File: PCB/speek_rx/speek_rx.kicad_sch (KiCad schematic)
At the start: 24 parts, among them U1 ESP32-D0WD-V3, U2 W25Q32JVSSIQ_C179173, X1 XL2EL89CPI-111YLC-40M

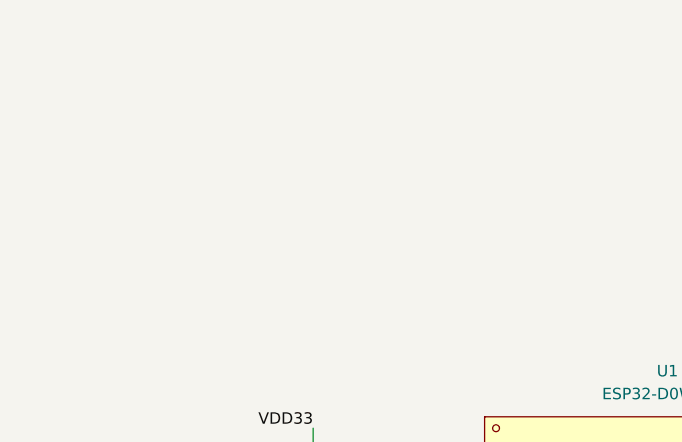
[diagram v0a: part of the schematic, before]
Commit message: finishs
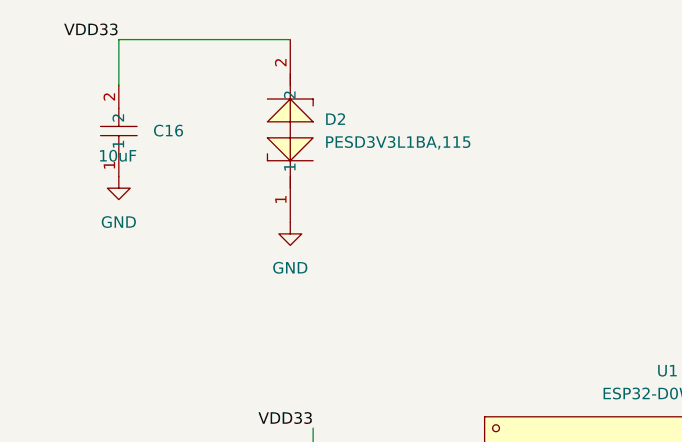
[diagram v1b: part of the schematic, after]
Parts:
- added C16: 10uF, lcsc:C0402, symbol lcsc:CL05A106MP5NUNC_C15525
- added D2: PESD3V3L1BA,115, easyeda2kicad:SOD-323_L1.7-W1.3-LS2.5-BI-1, symbol lcsc:PESD3V3L1BA,115
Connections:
- net GND: now also C16.1, D2.1
- net VDD33: now also C16.2, D2.2

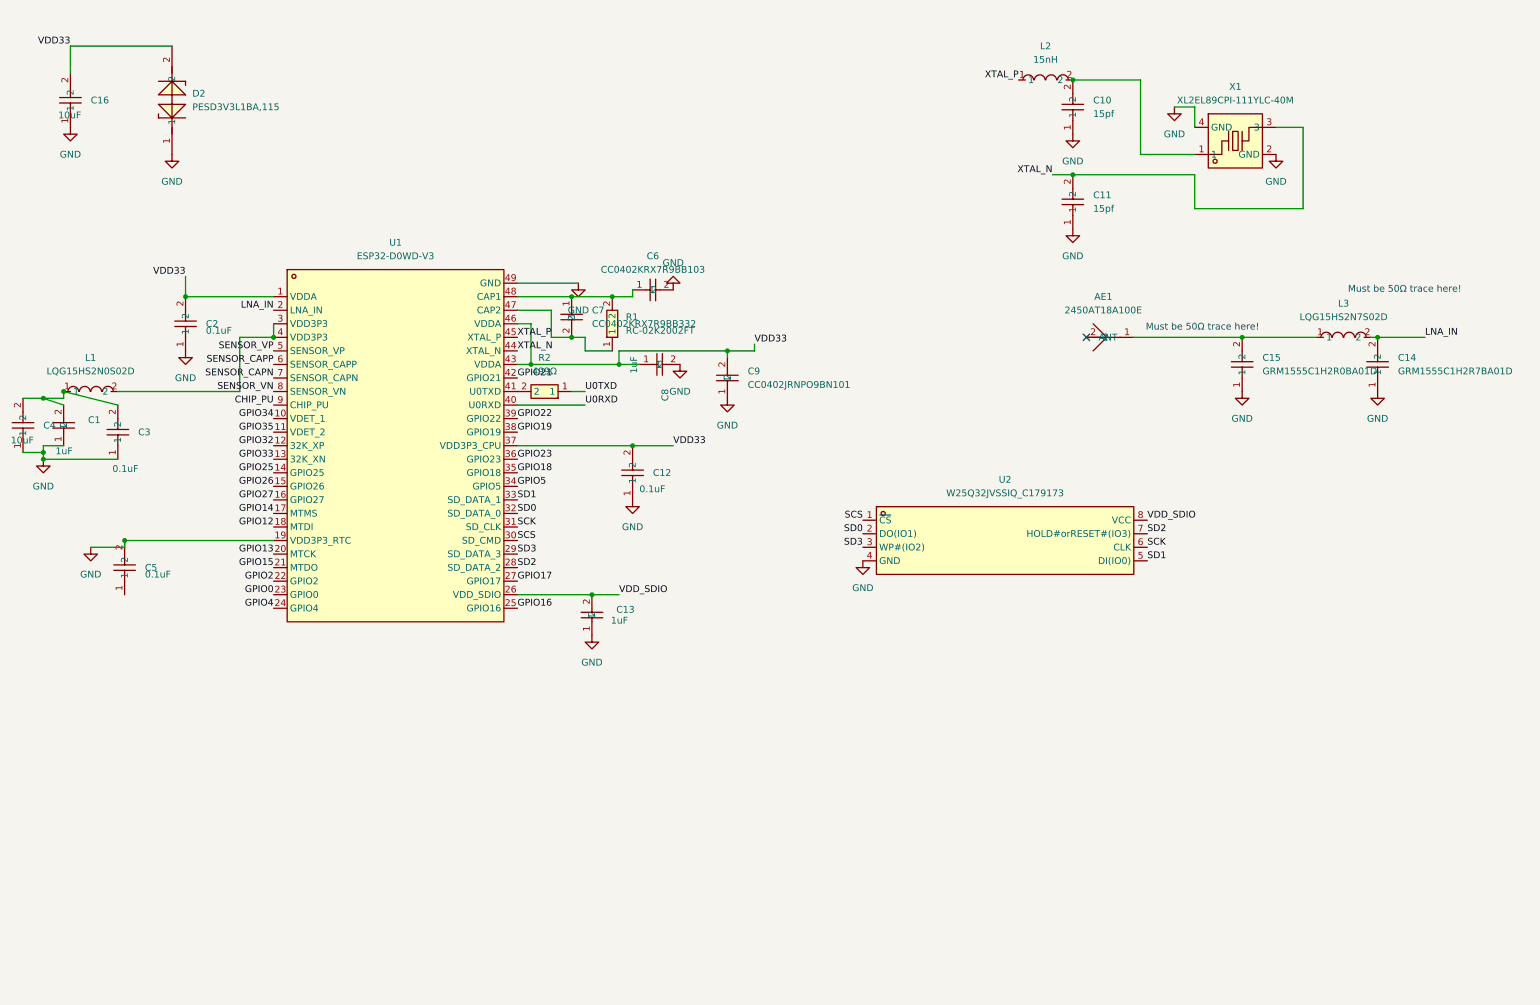
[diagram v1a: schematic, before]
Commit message: ldo, strappings, uart, USB
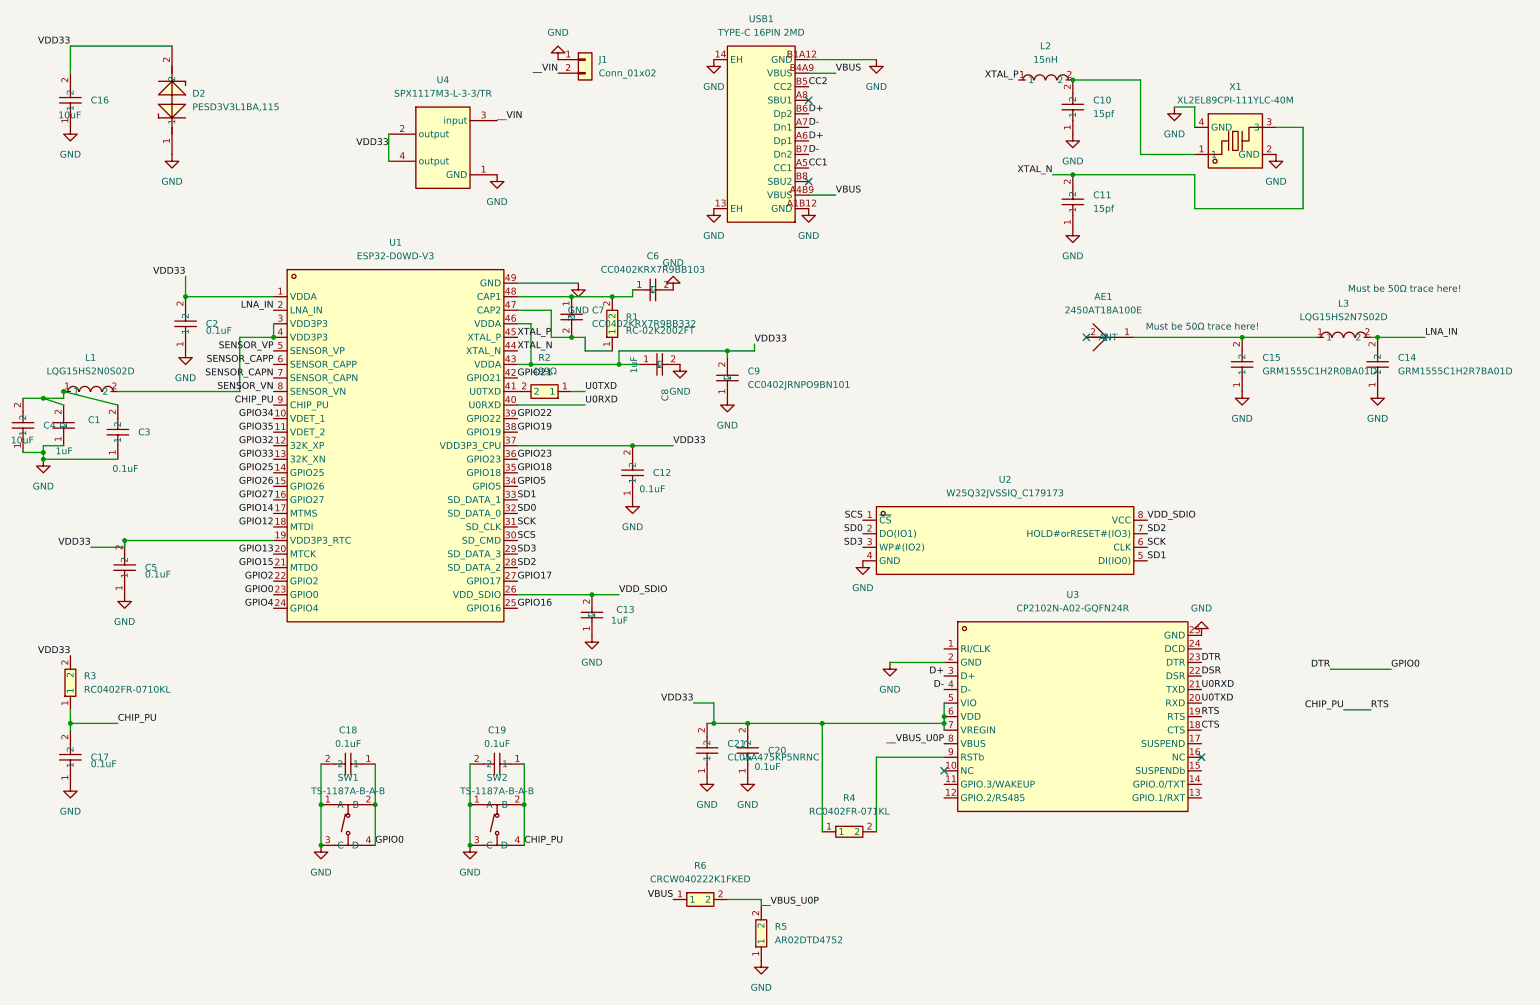
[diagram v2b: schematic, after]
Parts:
- added C17, C18, C19, C20: 0.1uF, lcsc:C0402, symbol lcsc:CC0402KRX7R7BB104
- added C21: CL05A475KP5NRNC, easyeda2kicad:C0402, symbol lcsc:CL05A475KP5NRNC
- added J1: Conn_01x02, symbol Connector_Generic:Conn_01x02
- added R3: RC0402FR-0710KL, easyeda2kicad:R0402, symbol lcsc:RC0402FR-0710KL
- added R4: RC0402FR-071KL, easyeda2kicad:R0402, symbol lcsc:RC0402FR-071KL
- added R5: AR02DTD4752, easyeda2kicad:R0402, symbol lcsc:AR02DTD4752
- added R6: CRCW040222K1FKED, easyeda2kicad:R0402, symbol lcsc:CRCW040222K1FKED
- added SW1, SW2: TS-1187A-B-A-B, easyeda2kicad:SW-SMD_4P-L5.1-W5.1-P3.70-LS6.5-TL_H1.5, symbol lcsc:TS-1187A-B-A-B
- added U3: CP2102N-A02-GQFN24R, easyeda2kicad:QFN-24_L4.0-W4.0-P0.50-TL-EP2.6, symbol lcsc:CP2102N-A02-GQFN24R
- added U4: SPX1117M3-L-3-3/TR, easyeda2kicad:SOT-223-4_L6.5-W3.5-P2.30-LS7.0-BR, symbol lcsc:SPX1117M3-L-3-3_TR
- added USB1: TYPE-C 16PIN 2MD, lcsc:USB-C-SMD_TYPE-C-16PIN-2MD-073, symbol lcsc:TYPE-C16PIN2MD
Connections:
- net CHIP_PU: now also C17.2, C19.1, R3.1, SW2.2 (B), SW2.4 (D), U3.19 (RTS)
- net GND: now also C5.1, C17.1, C18.2, C19.2, C20.1, C21.1, J1.1 (Pin_1), R5.1, SW1.1 (A), SW1.3 (C), SW2.1 (A), SW2.3 (C), U3.2 (GND), U3.25 (GND), U4.1 (GND), USB1.13 (EH), USB1.14 (EH), USB1.A1B12 (GND), USB1.B1A12 (GND); no longer C5.2, U1.19 (VDD3P3_RTC)
- net U0RXD: now also U3.21 (TXD)
- net U0TXD: now also U3.20 (RXD)
- net VDD33: now also C5.2, U1.19 (VDD3P3_RTC), C20.2, C21.2, R3.2, R4.1, U3.5 (VIO), U3.6 (VDD), U3.7 (VREGIN), U4.2 (output), U4.4 (output)
- net GPIO0 renamed DTR
- net DTR: now also C18.1, SW1.2 (B), SW1.4 (D), U3.23 (DTR)
- new net: R4.2, U3.9 (RSTb)
- new net CC1: USB1.A5 (CC1)
- new net CC2: USB1.B5 (CC2)
- new net CTS: U3.18 (CTS)
- new net D+: U3.3 (D+), USB1.A6 (Dp1), USB1.B6 (Dp2)
- new net D-: U3.4 (D-), USB1.A7 (Dn1), USB1.B7 (Dn2)
- new net DSR: U3.22 (DSR)
- new net VBUS: R6.1, USB1.A4B9 (VBUS), USB1.B4A9 (VBUS)
- new net __VBUS_U0P: R5.2, R6.2, U3.8 (VBUS)
- new net __VIN: J1.2 (Pin_2), U4.3 (input)
- no-connect marks 1 -> 5

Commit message: the speaker and stuff
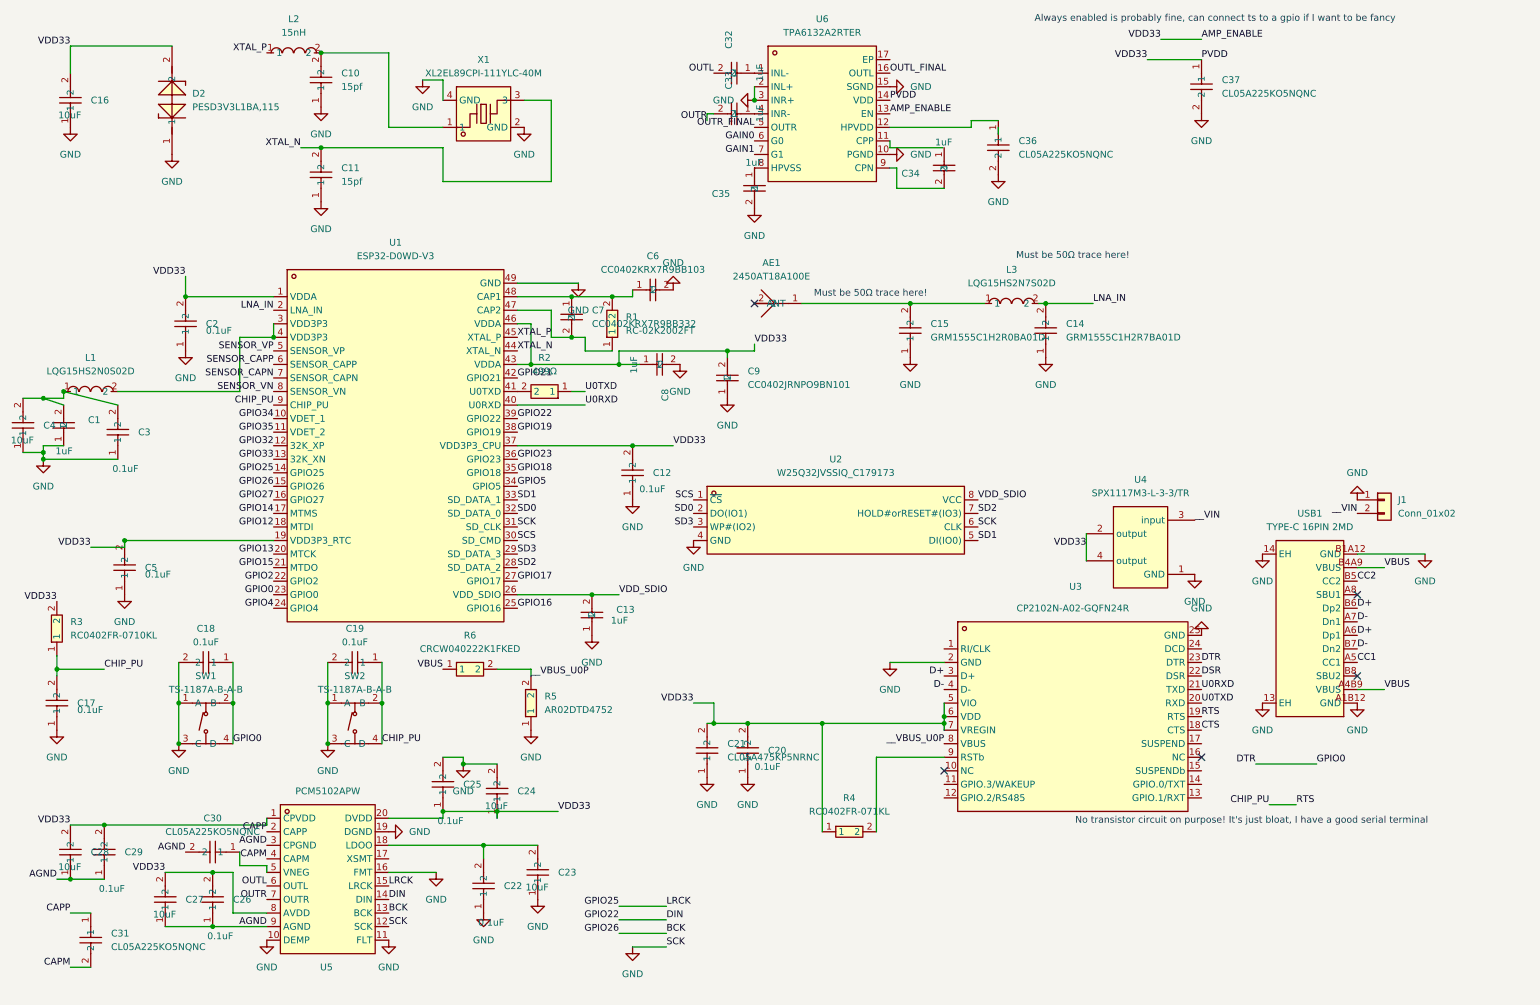
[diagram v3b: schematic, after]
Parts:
- added C22, C25, C26, C29: 0.1uF, lcsc:C0402, symbol lcsc:CC0402KRX7R7BB104
- added C23, C24, C27, C28: 10uF, lcsc:C0402, symbol lcsc:CL05A106MP5NUNC_C15525
- added C30, C31, C36, C37: CL05A225KO5NQNC, easyeda2kicad:C0402, symbol lcsc:CL05A225KO5NQNC
- added C32, C33, C34, C35: 1uF, lcsc:C0402, symbol lcsc:CL05A105KO5NNNC
- added U5: PCM5102APW, easyeda2kicad:TSSOP-20_L6.5-W4.4-P0.65-LS6.4-BL, symbol lcsc:PCM5102APW
- added U6: TPA6132A2RTER, easyeda2kicad:WQFN-16_L3.0-W3.0-P0.50-TL-EP1.6, symbol lcsc:TPA6132A2RTER
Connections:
- net SCK is gone; now on net GND: U1.31 (SD_CLK), U2.6 (CLK)
- net GND: now also C22.1, C23.1, C24.2, C25.2, C35.2, C36.2, C37.2, U5.10 (DEMP), U5.11 (FLT), U5.12 (SCK), U5.16 (FMT), U5.19 (DGND), U6.10 (PGND), U6.15 (SGND), U6.2 (INL+), U6.3 (INR+)
- net GPIO25: now also U5.15 (LRCK)
- net GPIO22 renamed DIN
- net DIN: now also U5.14 (DIN)
- net GPIO26 renamed BCK
- net BCK: now also U5.13 (BCK)
- net VDD33 renamed AMP_ENABLE
- net AMP_ENABLE: now also C24.1, C25.1, C26.2, C27.2, C28.2, C29.2, C37.1, U5.1 (CPVDD), U5.20 (DVDD), U5.8 (AVDD), U6.13 (EN), U6.14 (VDD)
- new net: C22.2, C23.2, U5.18 (LDOO)
- new net: C32.1, U6.1 (INL-)
- new net: C36.1, U6.12 (HPVDD)
- new net: C33.1, U6.4 (INR-)
- new net: C35.1, U6.8 (HPVSS)
- new net: C34.2, U6.9 (CPN)
- new net: C30.1, U5.5 (VNEG)
- new net AGND: C26.1, C27.1, C28.1, C29.1, C30.2, U5.3 (CPGND), U5.9 (AGND)
- new net CAPM: C31.2, U5.4 (CAPM)
- new net CAPP: C31.1, U5.2 (CAPP)
- new net GAIN0: U6.6 (G0)
- new net GAIN1: U6.7 (G1)
- new net OUTL: C32.2, U5.6 (OUTL)
- new net OUTL_FINAL: U6.16 (OUTL)
- new net OUTR: C33.2, U5.7 (OUTR)
- new net OUTR_FINAL: U6.5 (OUTR)
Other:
- note added: "Always enabled is probably fine, can connect ts to a gpio if I want to be fancy"
- note added: "No transistor circuit on purpose! It's just bloat, I have a good serial terminal"
- moved on the sheet: AE1, C10, C11, C14, C15, C17, C18, C19, J1, L2, L3, R3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
